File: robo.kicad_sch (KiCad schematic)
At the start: 7 parts, among them J1 Barrel_Jack_MountingPin, U1 L298N

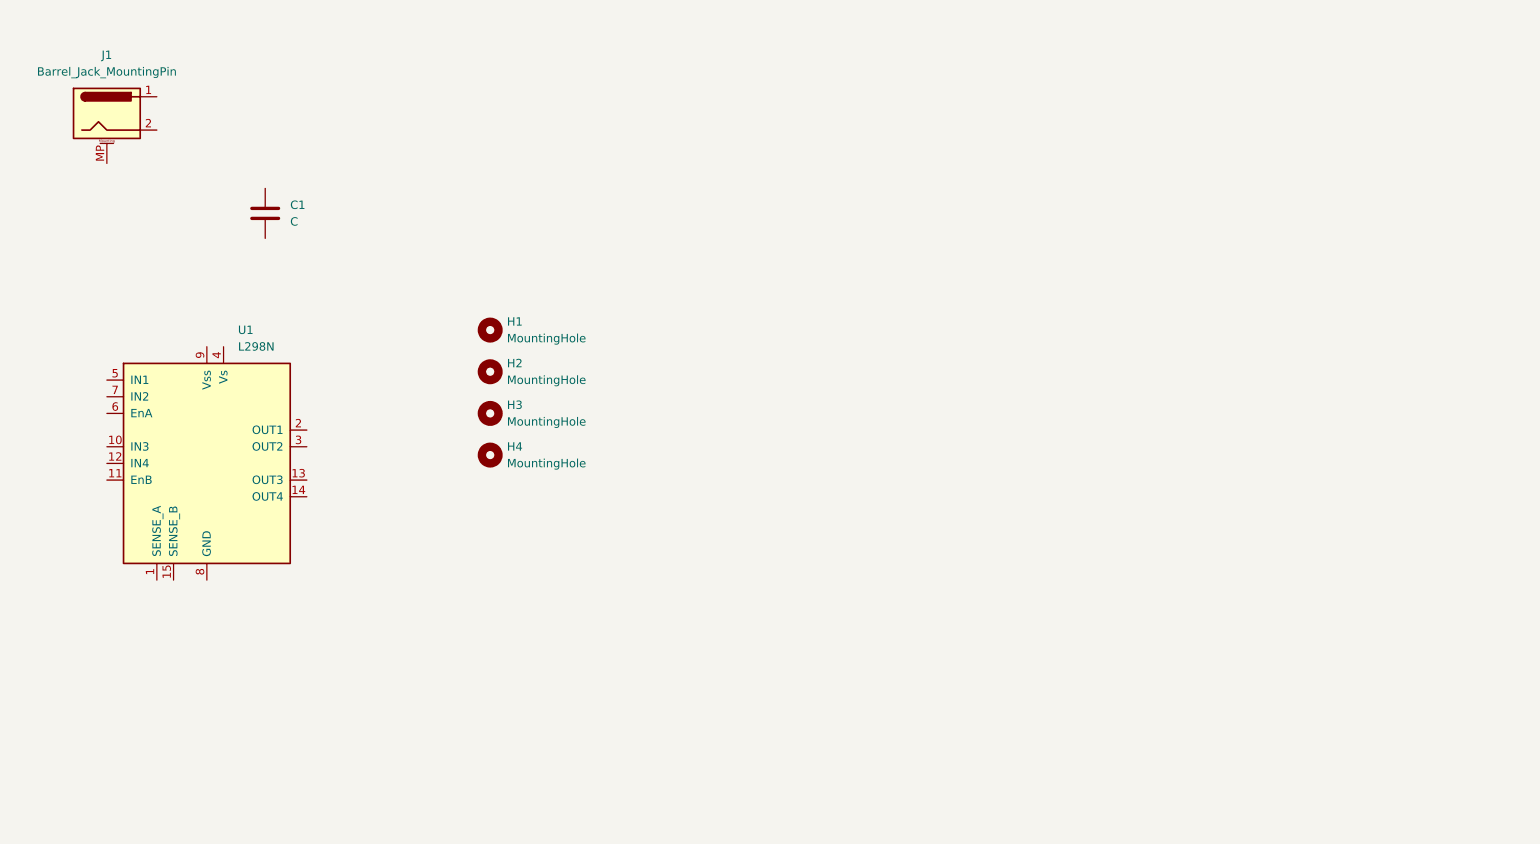
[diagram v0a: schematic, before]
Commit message: Testing testing 123
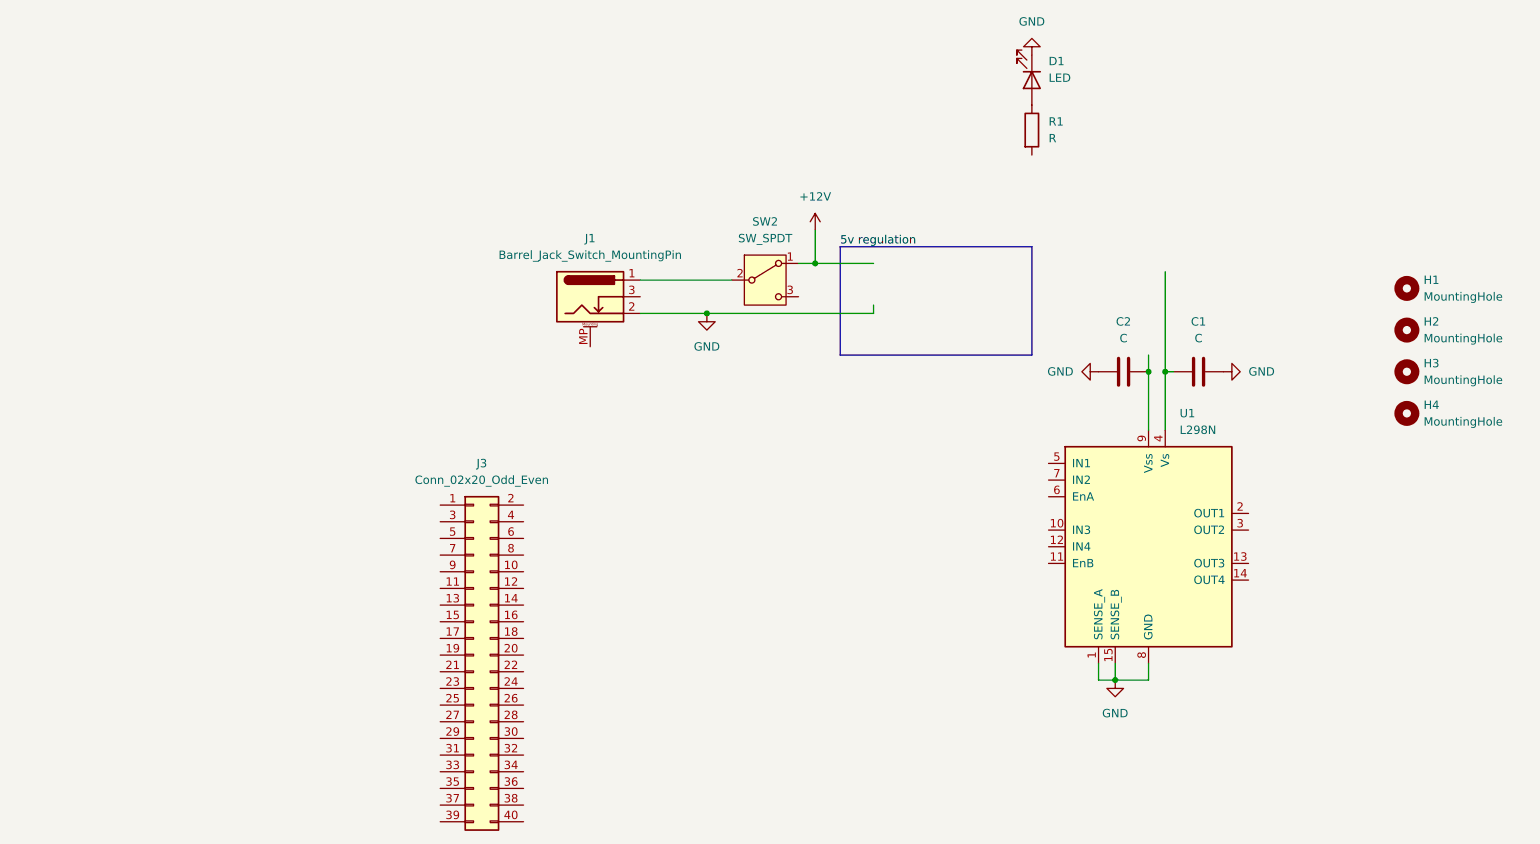
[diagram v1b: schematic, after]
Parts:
- removed J1: Barrel_Jack_MountingPin, symbol Connector:Barrel_Jack_MountingPin
- added C2: C, Capacitor_THT:C_Disc_D3.0mm_W1.6mm_P2.50mm, symbol Device:C
- added D1: LED, symbol Device:LED
- added J1: Barrel_Jack_Switch_MountingPin, Connector_BarrelJack:BarrelJack_Horizontal, symbol Connector:Barrel_Jack_Switch_MountingPin
- added J3: Conn_02x20_Odd_Even, symbol Connector_Generic:Conn_02x20_Odd_Even
- added R1: R, symbol Device:R
- added SW2: SW_SPDT, symbol Switch:SW_SPDT
- C1: footprint (none) -> Capacitor_THT:C_Disc_D3.0mm_W1.6mm_P2.50mm
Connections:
- net GND: now reaches U1.1 (SENSE_A)
- net GND: now also C1.2, U1.15 (SENSE_B), U1.8 (GND), C2.1, D1.1 (K), J1.2
- net at U1.4 (Vs): now also C1.1
- net at U1.9 (Vss): now also C2.2
- new net: D1.2 (A), R1.1
- new net: J1.1, SW2.2 (B)
- new net +12V: SW2.1 (A)
